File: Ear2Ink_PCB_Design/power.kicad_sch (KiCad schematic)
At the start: 20 parts, among them P1 OSTTE020104, U2 TPS562208DDCR, U3 AZ1117-3.3, U4 LM66100DCK, U5 LM66100DCK

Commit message: footprints
missing L tho
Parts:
- C11, C12, C13, C16, C17: footprint (none) -> Capacitor_SMD:C_0603_1608Metric_Pad1.08x0.95mm_HandSolder
- D1, D2: footprint (none) -> Resistor_SMD:R_0805_2012Metric_Pad1.20x1.40mm_HandSolder
- U2: footprint DDC0006A_N -> Buck:DDC0006A_N
- U3: footprint (none) -> LDO:SOT-223_DIO
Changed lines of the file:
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@@
 			)
 		)
-		(property "Footprint" ""
+		(property "Footprint" "Capacitor_SMD:C_0603_1608Metric_Pad1.08x0.95mm_HandSolder"
 			(at 111.76 117.1448 0)
 			(effects
@@
 			)
 		)
-		(property "Footprint" ""
+		(property "Footprint" "Resistor_SMD:R_0805_2012Metric_Pad1.20x1.40mm_HandSolder"
 			(at 109.22 72.39 0)
 			(effects
@@
 			)
 		)
-		(property "Footprint" ""
+		(property "Footprint" "Capacitor_SMD:C_0603_1608Metric_Pad1.08x0.95mm_HandSolder"
 			(at 74.6252 48.26 0)
 			(effects
@@
 			)
 		)
-		(property "Footprint" ""
+		(property "Footprint" "Resistor_SMD:R_0805_2012Metric_Pad1.20x1.40mm_HandSolder"
 			(at 187.96 143.51 0)
 			(effects
@@
 			)
 		)
-		(property "Footprint" "DDC0006A_N"
+		(property "Footprint" "Buck:DDC0006A_N"
 			(at 78.74 120.65 0)
 			(effects
@@
 			)
 		)
-		(property "Footprint" ""
+		(property "Footprint" "LDO:SOT-223_DIO"
 			(at 60.96 33.02 0)
 			(effects
@@
 			)
 		)
-		(property "Footprint" ""
+		(property "Footprint" "Capacitor_SMD:C_0603_1608Metric_Pad1.08x0.95mm_HandSolder"
 			(at 148.2852 125.73 0)
 			(effects
@@
 			)
 		)
-		(property "Footprint" ""
+		(property "Footprint" "Capacitor_SMD:C_0603_1608Metric_Pad1.08x0.95mm_HandSolder"
 			(at 40.3352 48.26 0)
 			(effects
@@
 			)
 		)
-		(property "Footprint" ""
+		(property "Footprint" "Capacitor_SMD:C_0603_1608Metric_Pad1.08x0.95mm_HandSolder"
 			(at 39.6748 119.38 0)
 			(effects

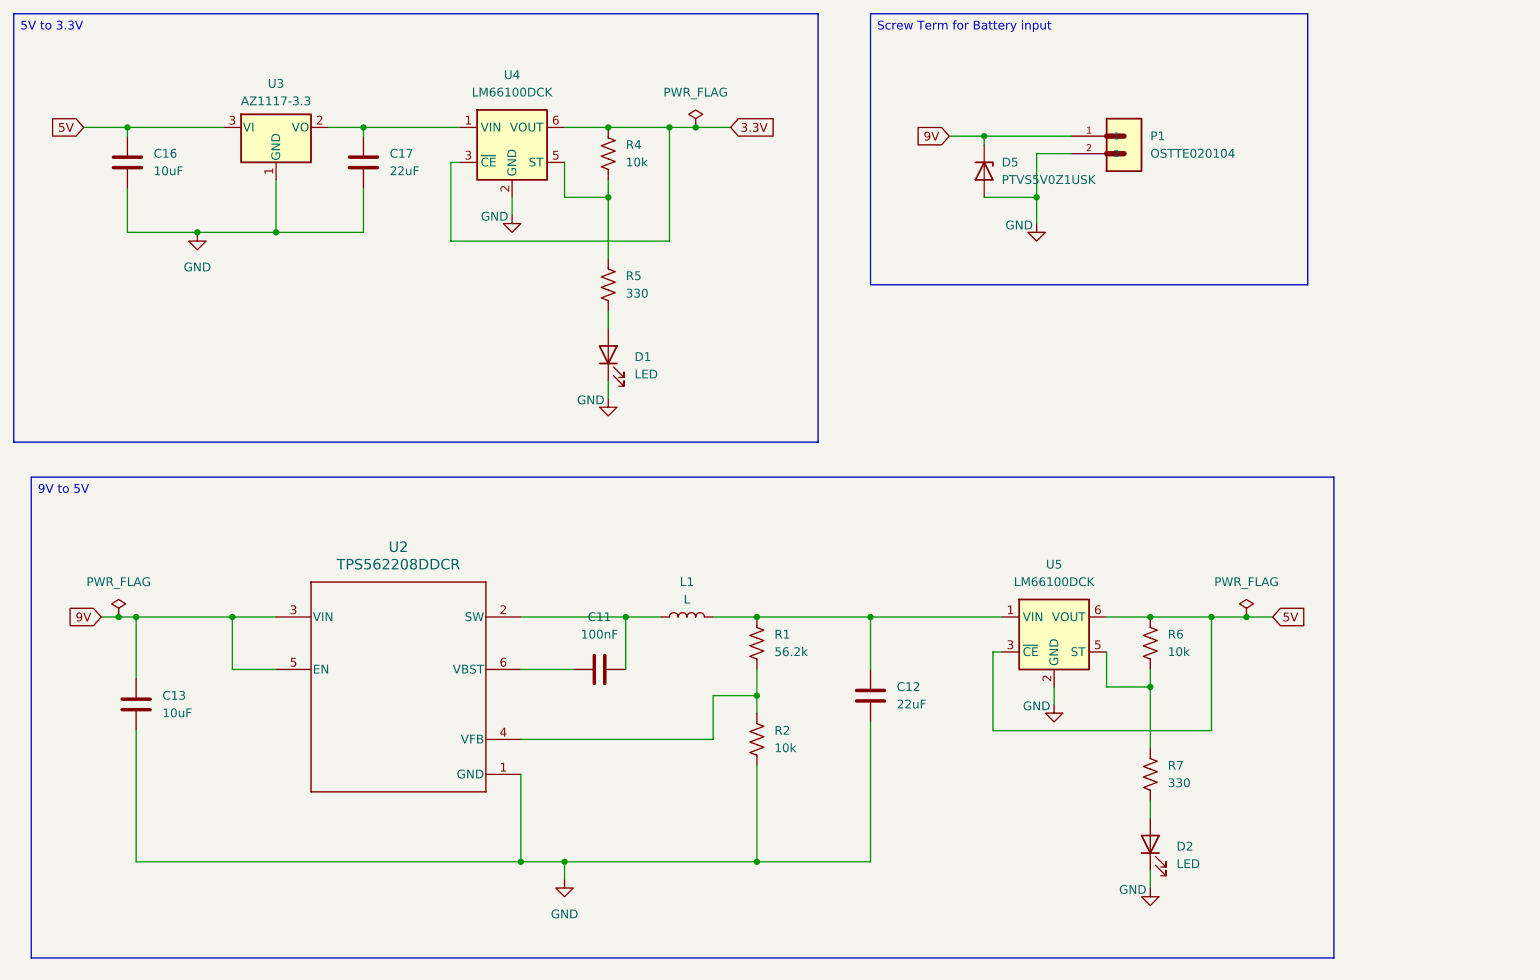
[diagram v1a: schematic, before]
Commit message: all footprints done
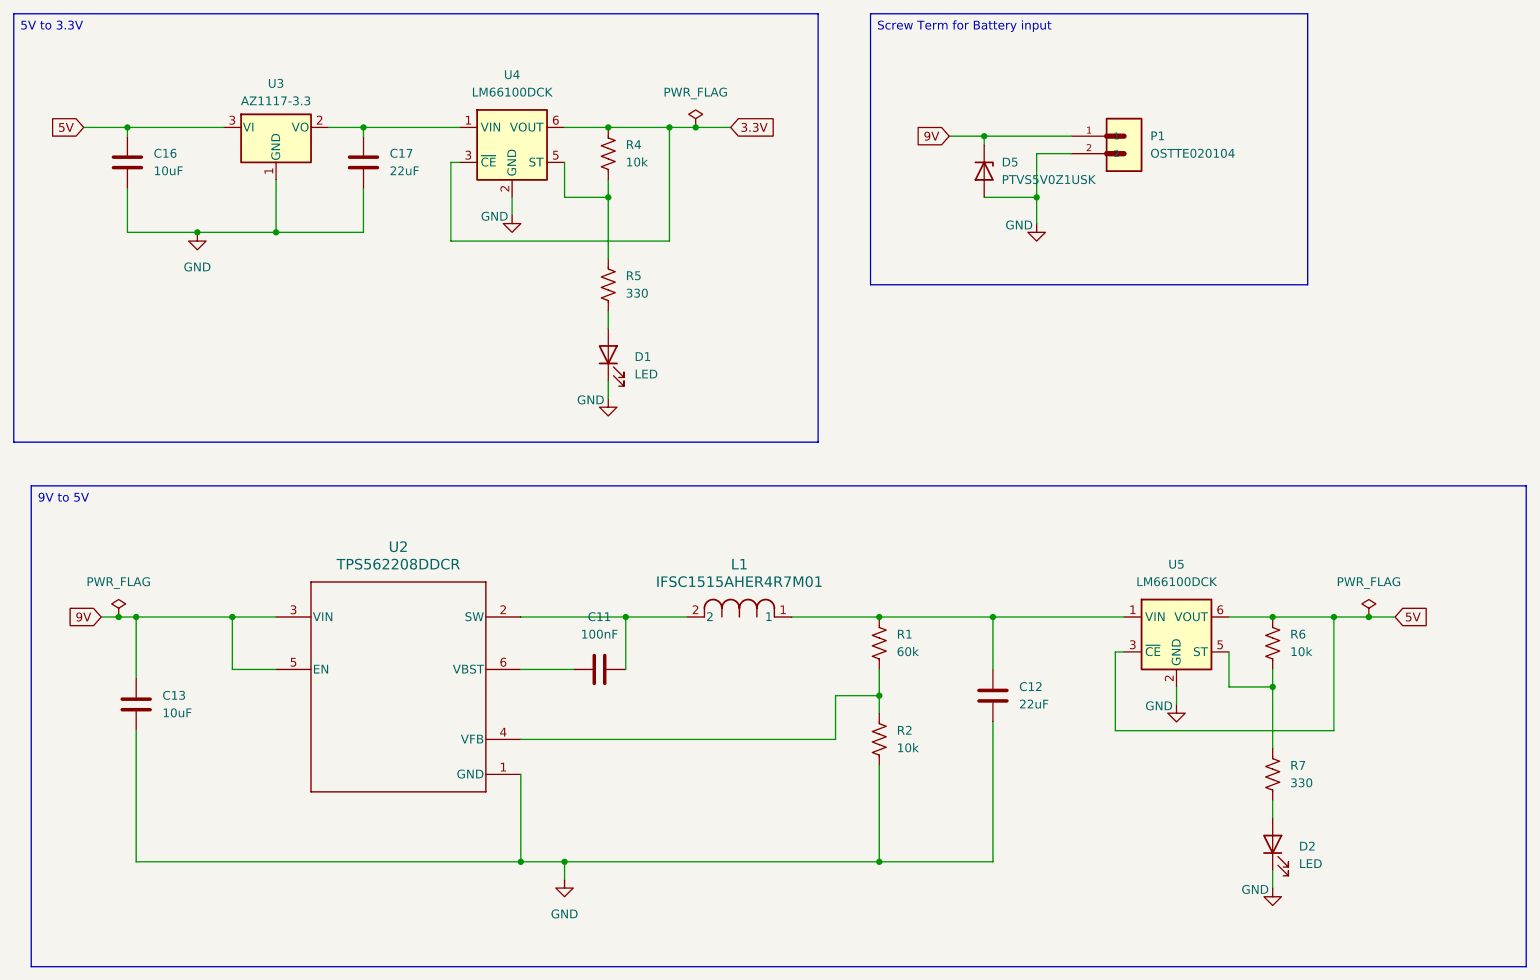
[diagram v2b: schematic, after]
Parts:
- removed L1: L, symbol Device:L
- added L1: IFSC1515AHER4R7M01, Inductor_SMD:L_Vishay_IFSC-1515AH_4x4x1.8mm, symbol Inductor:IFSC1515AHER4R7M01
- R1: value 56.2k -> 60k
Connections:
- net at C11.2, U2.2 (SW): now also L1.2
- net at C12.1, R1.1, U5.1 (VIN): now also L1.1
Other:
- moved on the sheet: C12, D2, R1, R2, R6, R7, U5
